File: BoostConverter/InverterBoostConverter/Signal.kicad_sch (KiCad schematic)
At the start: 58 parts, among them IC4 LM358DR, IC5 LM358DR, IC6 MCP2515-e_ST, IC7 TJA1050T_CM,118, SW1 SW_Push, U2 TL431AIDBZR, U4 TMP36xS, U5 TMP36xS, Y1 8MHz

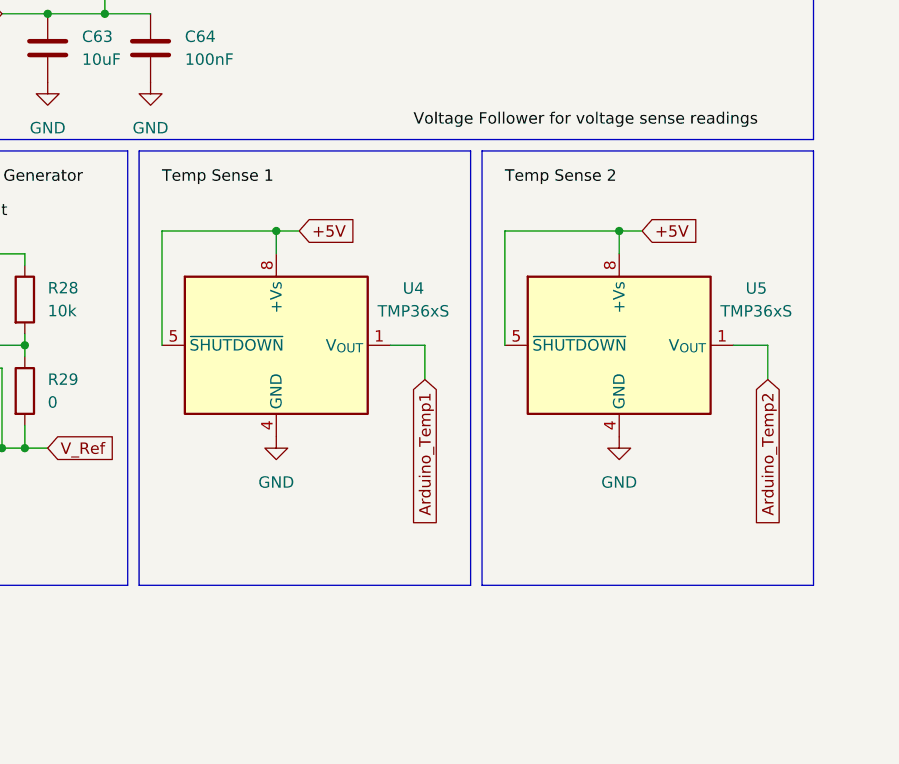
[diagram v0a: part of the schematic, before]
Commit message: Update boost converter layout
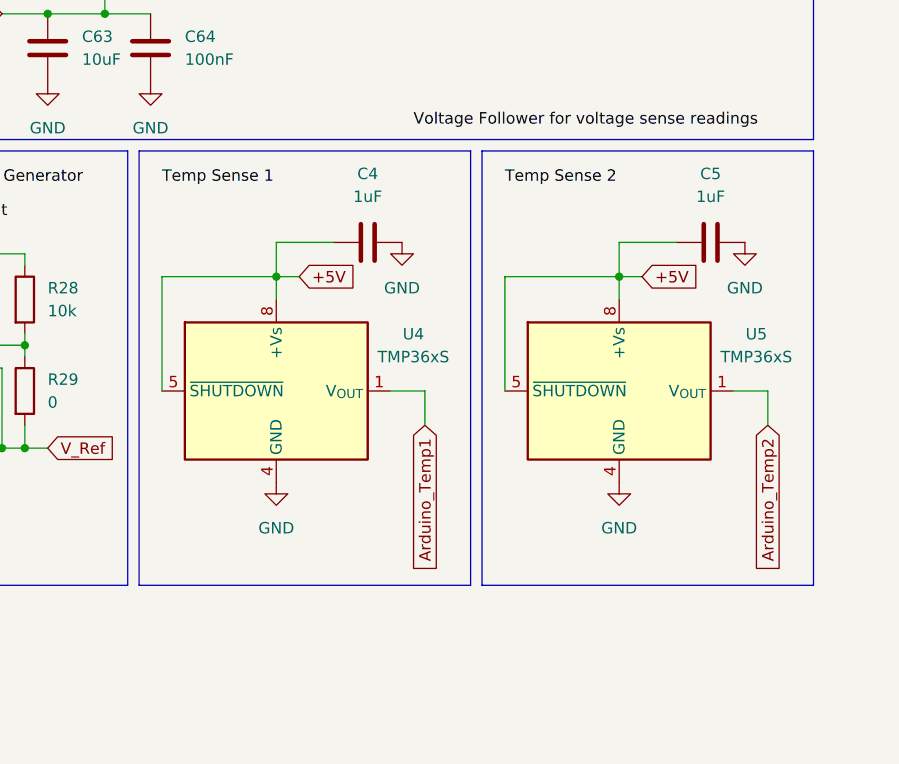
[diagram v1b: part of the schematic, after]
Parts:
- added C4, C5: 1uF, Capacitor_SMD:C_1210_3225Metric_Pad1.33x2.70mm_HandSolder, symbol Device:C
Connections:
- net +5V: now also C4.1, C5.1
- net GND: now also C4.2, C5.2
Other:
- moved on the sheet: U4, U5

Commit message: udpate
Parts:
- R70, R77: value 1M -> RC2512JK-071ML
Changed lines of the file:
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@@
 			)
 		)
-		(property "Value" "1M"
+		(property "Value" "RC2512JK-071ML"
 			(at 259.0801 50.8 90)
 			(effects
@@
 			)
 		)
-		(property "Value" "1M"
+		(property "Value" "RC2512JK-071ML"
 			(at 227.3301 50.8 90)
 			(effects
